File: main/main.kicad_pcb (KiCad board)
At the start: 4 copper layers, 166.6 x 111.3 mm, 156 parts, among them IC1 TPS54294PWP, IC2 TPS54294PWP, IC3 ESP-PSRAM64H, IC4 PCM1741E, J1 STX-3000, J2 DIN-5_180degree, J3 Barrel_Jack_Switch_Pin3Ring, J4 FPGA_debug, J5 FPGA_GPIO, J6 MCU_debug, J7 MCU_GPIO, J8 BACKUP_SPI, J9 Breakout I2S, SW1 FBKey, SW2 FBKey, SW3 FBKey, SW4 FBKey, SW5 FBKey, U1 6N138, U2 S25FL127S, U3 XC7A100T-FTG256, U4 EFM32GG12B810F1024GQ64, U5 Opamp_Dual_Generic, X1 FGPA_Oscillator, X2 MCU_Oscillator

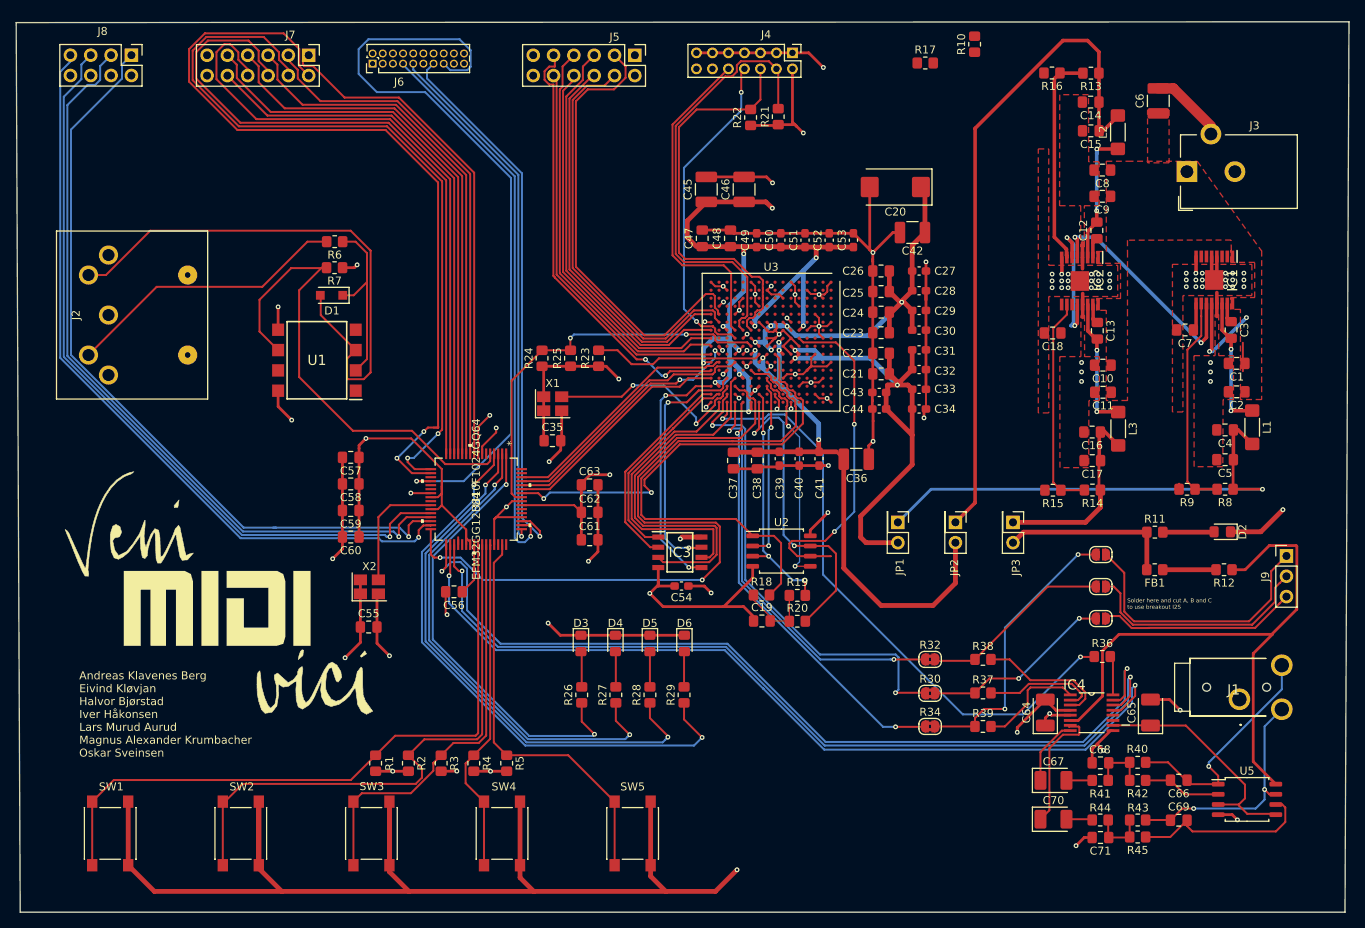
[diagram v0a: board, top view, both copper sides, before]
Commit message: Finished (?) board
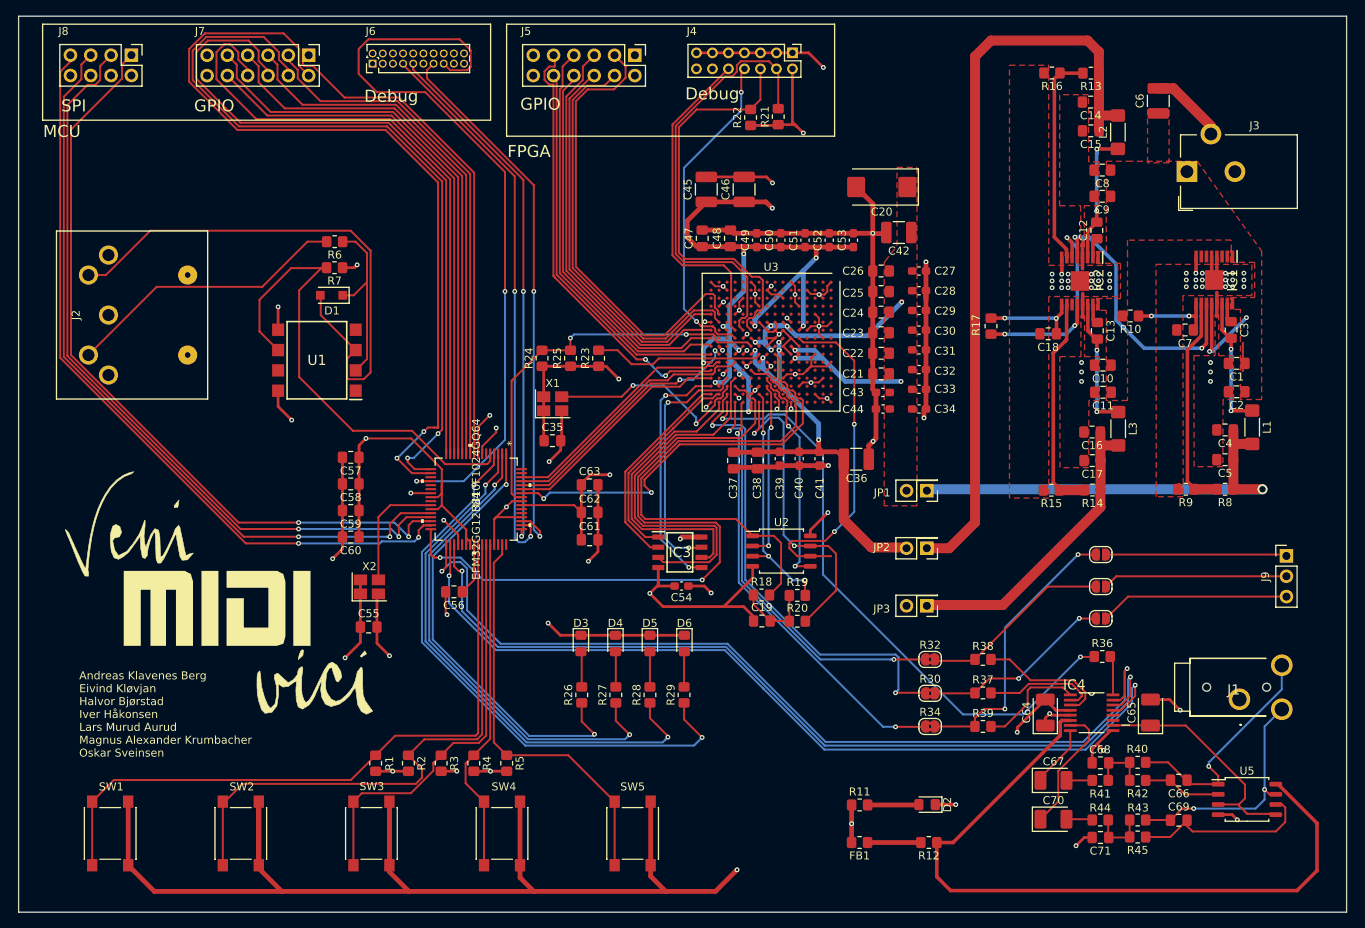
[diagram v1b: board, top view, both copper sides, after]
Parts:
- moved D2 50.2 mm to (184.6, 146.6)
- moved FB1 50.2 mm to (176.1, 151.3)
- moved R11 50.2 mm to (176.1, 146.6)
- moved R12 50.2 mm to (184.8, 151.3)
- moved R10 39.2 mm to (210.0, 85.5), turned to 180 degrees
- moved R17 33.9 mm to (192.6, 86.7), turned to 270 degrees
- moved JP3 15.0 mm to (184.5, 121.7), turned to 180 degrees
- moved JP1 5.37 mm to (184.5, 107.3), turned to 180 degrees
- moved JP2 4.82 mm to (184.5, 114.5), turned to 180 degrees
- moved C20 1.70 mm to (178.9, 69.4)
- moved C42 1.70 mm to (181.0, 75.0)
- moved C18 0.56 mm to (199.7, 87.7)
- moved C43 0.45 mm to (179.0, 95.0)
- moved C44 0.45 mm to (179.0, 97.1)
- moved R15 0.19 mm to (200.1, 107.2)
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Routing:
- net +1V0: track 126.6 -> 51.1 mm
- net +1V8: track 76.7 -> 57.8 mm
- net +3V3: track 403.0 -> 385.8 mm, vias 24 -> 25
- net +3.3VA: track 75.6 -> 90.6 mm
- net Net-(C16-Pad1): track 24.4 -> 38.5 mm
- net Net-(C18-Pad1): track 0.00 -> 12.1 mm, vias 0 -> 2
- net Net-(J9-Pad1): track 34.3 -> 22.6 mm
- net Net-(C14-Pad1): track 84.7 -> 96.0 mm
- net Net-(IC2-Pad12): track 17.5 -> 28.0 mm, vias 2 -> 3
- net Net-(C7-Pad1): track 3.37 -> 11.4 mm, vias 0 -> 2
- net Net-(J9-Pad2): track 29.5 -> 23.1 mm
- net Net-(C4-Pad1): track 61.5 -> 55.5 mm
- net Net-(IC1-Pad11): track 29.1 -> 34.2 mm
- net GND: track 373.4 -> 368.5 mm, vias 94 -> 95
- net Net-(J9-Pad3): track 24.9 -> 23.7 mm
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- added copper zone on F.Cu, net +1V0
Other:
- board size 166.6 x 111.3 mm -> 166 x 112 mm
- board text added: "Debug"
- board text added: "FPGA"
- board text added: "GPIO"
- board text added: "MCU"
- board text added: "SPI"
- board text removed: "Solder here and cut A, B and C to use breakout I2S"
